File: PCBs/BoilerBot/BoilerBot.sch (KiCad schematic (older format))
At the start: 24 parts, among them J1 Screw_Terminal_01x02, J10 Conn_01x03_Male, J2 Screw_Terminal_01x03, J3 Screw_Terminal_01x03, J4 Screw_Terminal_01x02, J5 Conn_01x05_Male, J6 Conn_01x03_Male, J7 Conn_01x03_Male, J8 Screw_Terminal_01x03, J9 Conn_01x04_Male, K1 ADW11, Q1 2N7002, Q2 2N7002, U1 AZ1117-5.0, U2 TB67H451FNG,EL

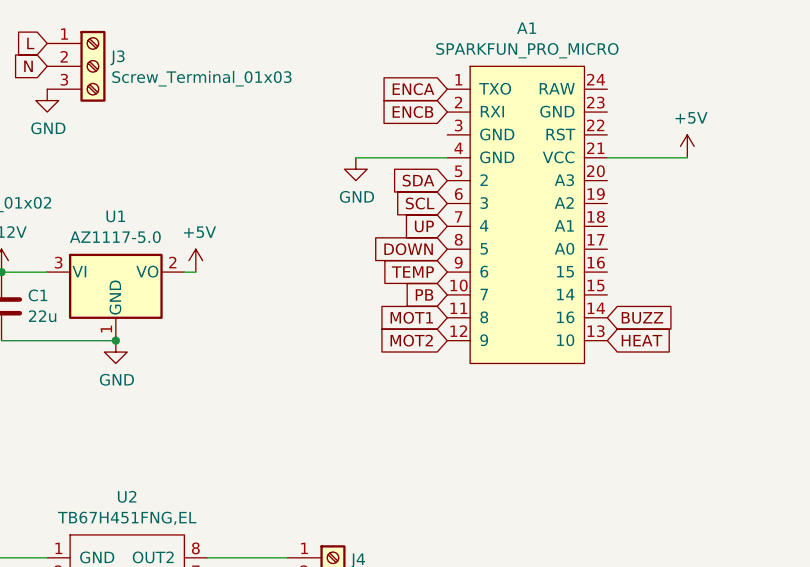
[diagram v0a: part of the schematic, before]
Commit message: PCBs ready to order
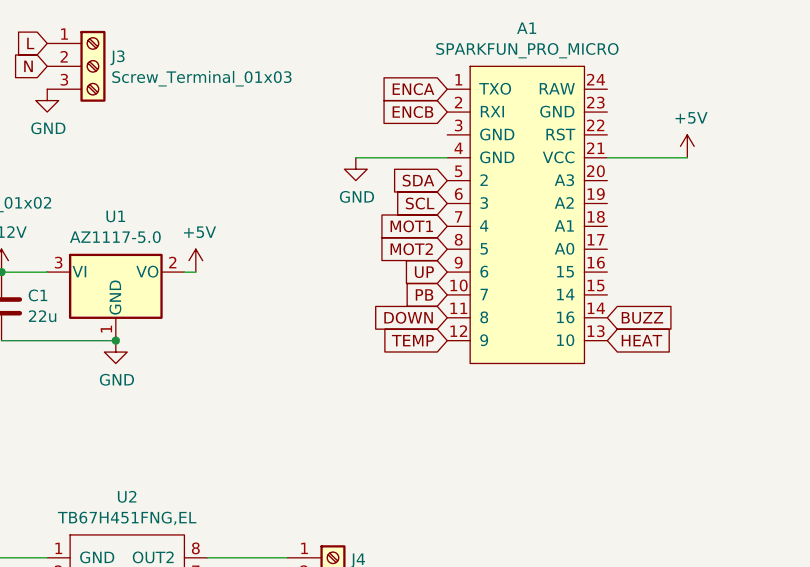
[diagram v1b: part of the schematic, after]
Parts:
- C3: footprint Capacitor_SMD:C_0805_2012Metric_Pad1.18x1.45mm_HandSolder -> Capacitor_SMD:CP_Elec_6.3x7.7
- K1: footprint Relay_THT:Relay_1P1T_NO_10x24x18.8mm_Panasonic_ADW11xxxxW_THT -> BoilerBot:OMRON_G5PZ-1A
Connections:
- net DOWN: now also A1.11 (8); no longer A1.8 (5)
- net MOT1: now also A1.7 (4); no longer A1.11 (8)
- net MOT2: now also A1.8 (5); no longer A1.12 (9)
- net TEMP: now also A1.12 (9); no longer A1.9 (6)
- net UP: now also A1.9 (6); no longer A1.7 (4)
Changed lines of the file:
@@
 Text GLabel 5200 3800 0    50   Input ~ 0
 SCL
+Text GLabel 5200 4100 0    50   Input ~ 0
+UP
+Text GLabel 5200 4300 0    50   Input ~ 0
+DOWN
 Text GLabel 5200 3900 0    50   Input ~ 0
-UP
+MOT1
 Text GLabel 5200 4000 0    50   Input ~ 0
-DOWN
-Text GLabel 5200 4300 0    50   Input ~ 0
-MOT1
+MOT2
 Text GLabel 5200 4400 0    50   Input ~ 0
-MOT2
-Text GLabel 5200 4100 0    50   Input ~ 0
 TEMP
 Text GLabel 5900 4400 2    50   Input ~ 0
@@
 F 0 "C3" H 4668 5946 50  0000 L CNN
 F 1 "100U" H 4668 5855 50  0000 L CNN
-F 2 "Capacitor_SMD:C_0805_2012Metric_Pad1.18x1.45mm_HandSolder" H 4588 5750 50  0001 C CNN
+F 2 "Capacitor_SMD:CP_Elec_6.3x7.7" H 4588 5750 50  0001 C CNN
 F 3 "~" H 4550 5900 50  0001 C CNN
 	1    4550 5900
@@
 F 0 "K1" H 6680 1896 50  0000 L CNN
 F 1 "ADW11" H 6680 1805 50  0000 L CNN
-F 2 "Relay_THT:Relay_1P1T_NO_10x24x18.8mm_Panasonic_ADW11xxxxW_THT" H 7575 1800 50  0001 C CNN
+F 2 "BoilerBot:OMRON_G5PZ-1A" H 7575 1800 50  0001 C CNN
 F 3 "https://www.panasonic-electric-works.com/pew/es/downloads/ds_dw_hl_en.pdf" H 6250 1850 50  0001 C CNN
 	1    6250 1850
